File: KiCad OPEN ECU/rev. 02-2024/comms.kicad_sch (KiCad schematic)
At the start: 9 parts, among them U19 MCP2562-E-SN, U4 AHT20, U5 BMP280

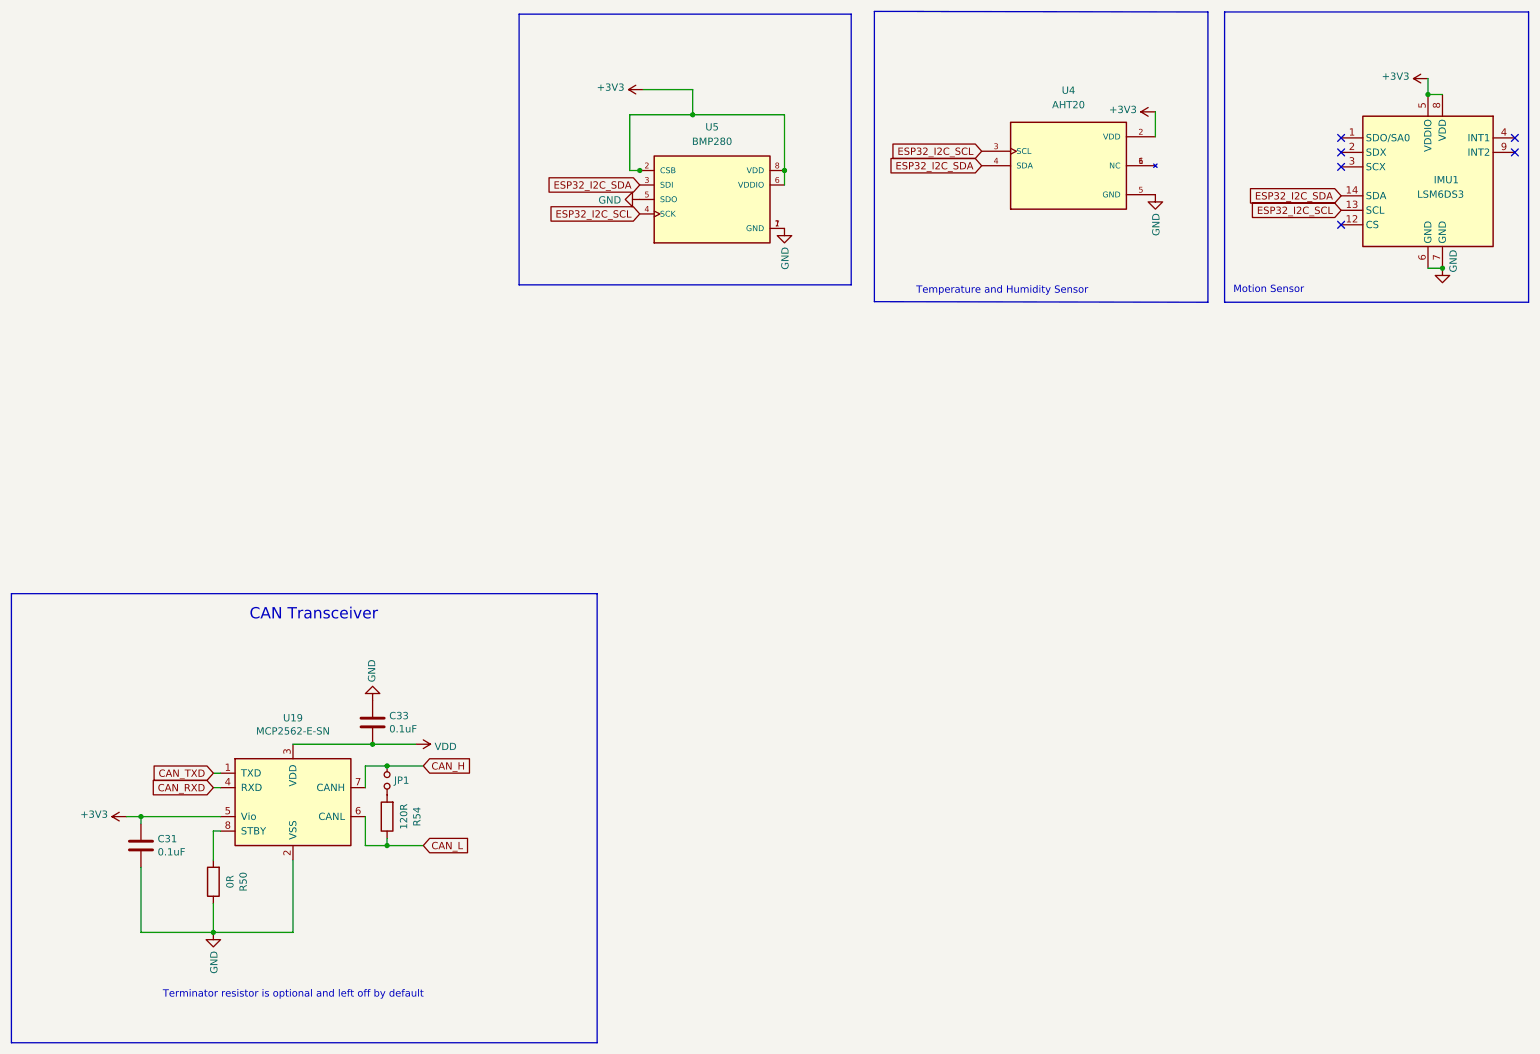
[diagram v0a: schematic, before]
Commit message: update
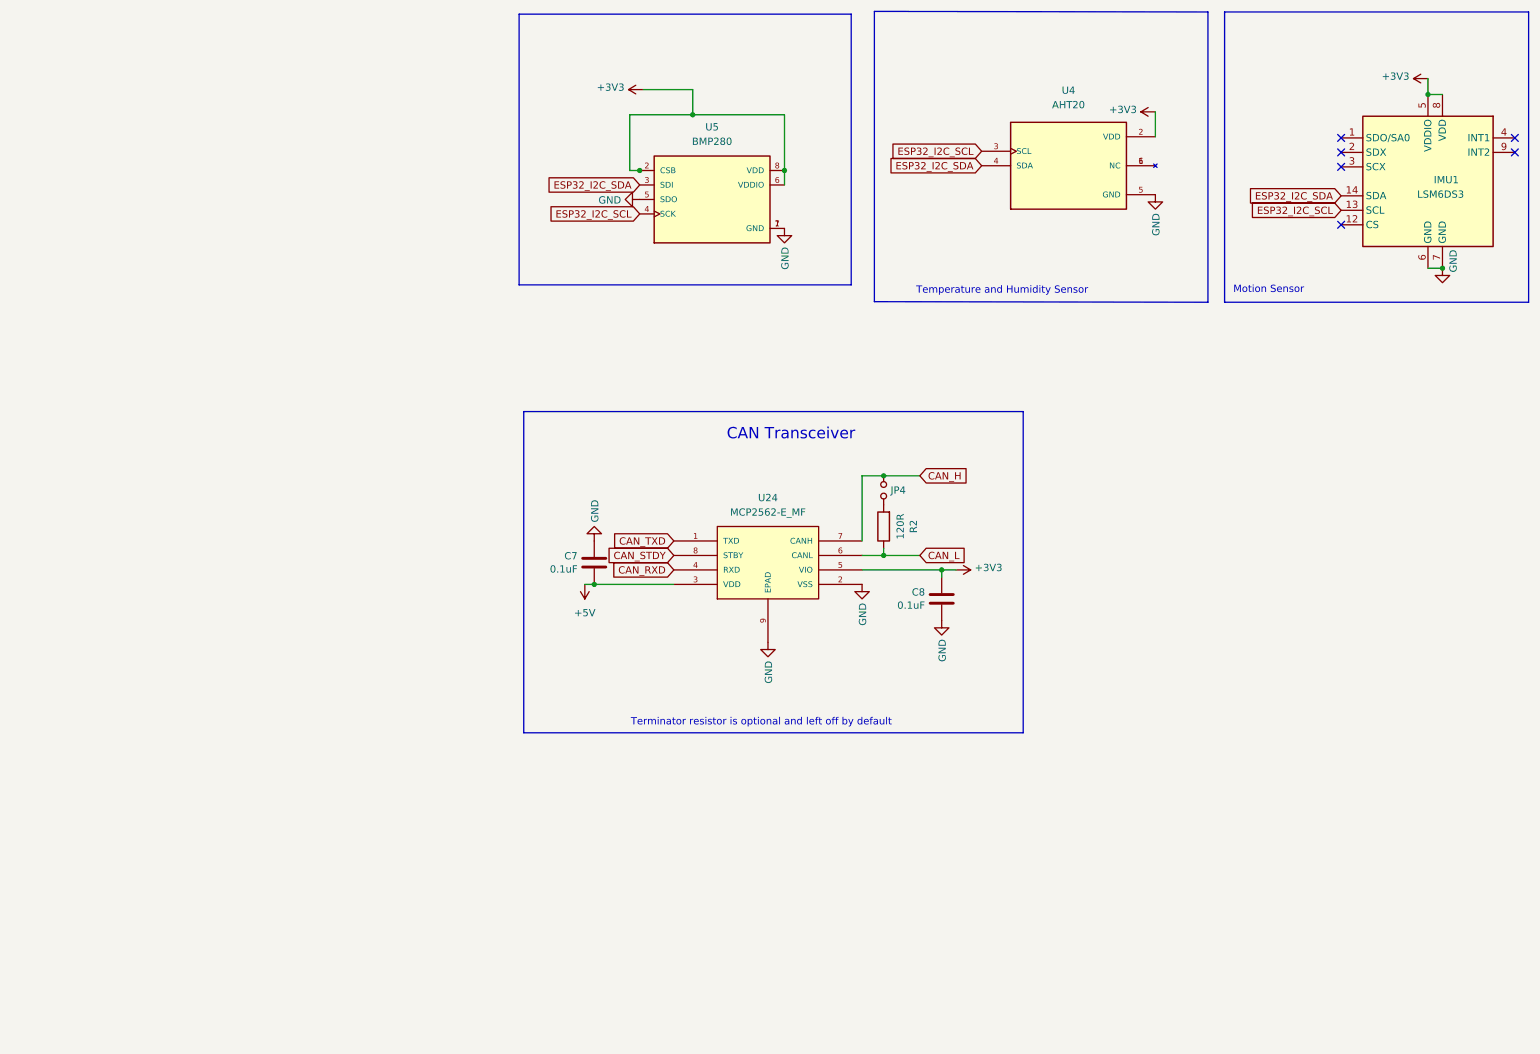
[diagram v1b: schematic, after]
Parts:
- removed C31, C33: 0.1uF, Capacitor_SMD:C_0805_2012Metric, symbol Device:C
- removed JP1: Jumper_NO_Small, Jumper:SolderJumper-2_P1.3mm_Open_Pad1.0x1.5mm, symbol Device:Jumper_NO_Small
- removed R50: 0R, Resistor_SMD:R_0805_2012Metric, symbol Device:R
- removed R54: 120R, Resistor_SMD:R_0805_2012Metric, symbol Device:R
- removed U19: MCP2562-E-SN, Package_SO:SOIC-8_3.9x4.9mm_P1.27mm, symbol Interface_CAN_LIN:MCP2562-E-SN
- added C7, C8: 0.1uF, Capacitor_SMD:C_0805_2012Metric, symbol Device:C
- added JP4: Jumper_NO_Small, Jumper:SolderJumper-2_P1.3mm_Open_Pad1.0x1.5mm, symbol Device:Jumper_NO_Small
- added R2: 120R, Resistor_SMD:R_0805_2012Metric, symbol Device:R
- added U24: MCP2562-E_MF, AeonLabs_Automotive:MCP2562 DFN, symbol AeonLabs_Automotive:MCP2562-E_MF
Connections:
- net +3V3: now also C8.1, U24.5 (VIO)
- net CAN_H: now also JP4.1, U24.7 (CANH)
- net CAN_L: now also R2.1, U24.6 (CANL)
- net CAN_RXD: now also U24.4 (RXD)
- net CAN_TXD: now also U24.1 (TXD)
- net GND: now also C7.1, C8.2, U24.2 (VSS), U24.9 (EPAD)
- new net: JP4.2, R2.2
- new net +5V: C7.2, U24.3 (VDD)
- new net CAN_STDY: U24.8 (STBY)
